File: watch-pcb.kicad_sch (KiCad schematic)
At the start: 104 parts, among them J2 Micro_SD_Card, J3 Conn_01x06_Socket, J4 USB_C_Receptacle, J5 ESP_ANT, U1 LIS3MDL, U10 MX25LM51245GXDI00, U2 BQ25629RYKR, U3 DRV2605LYZFR, U4 BQ27427YZFR, U5 APS12808L-3OBMx, U6 MAX30102, U7 LSM6DSV16XTR, U8 ESP32-S3, Y1 40MHz(10ppm), Y2 32.768kHz

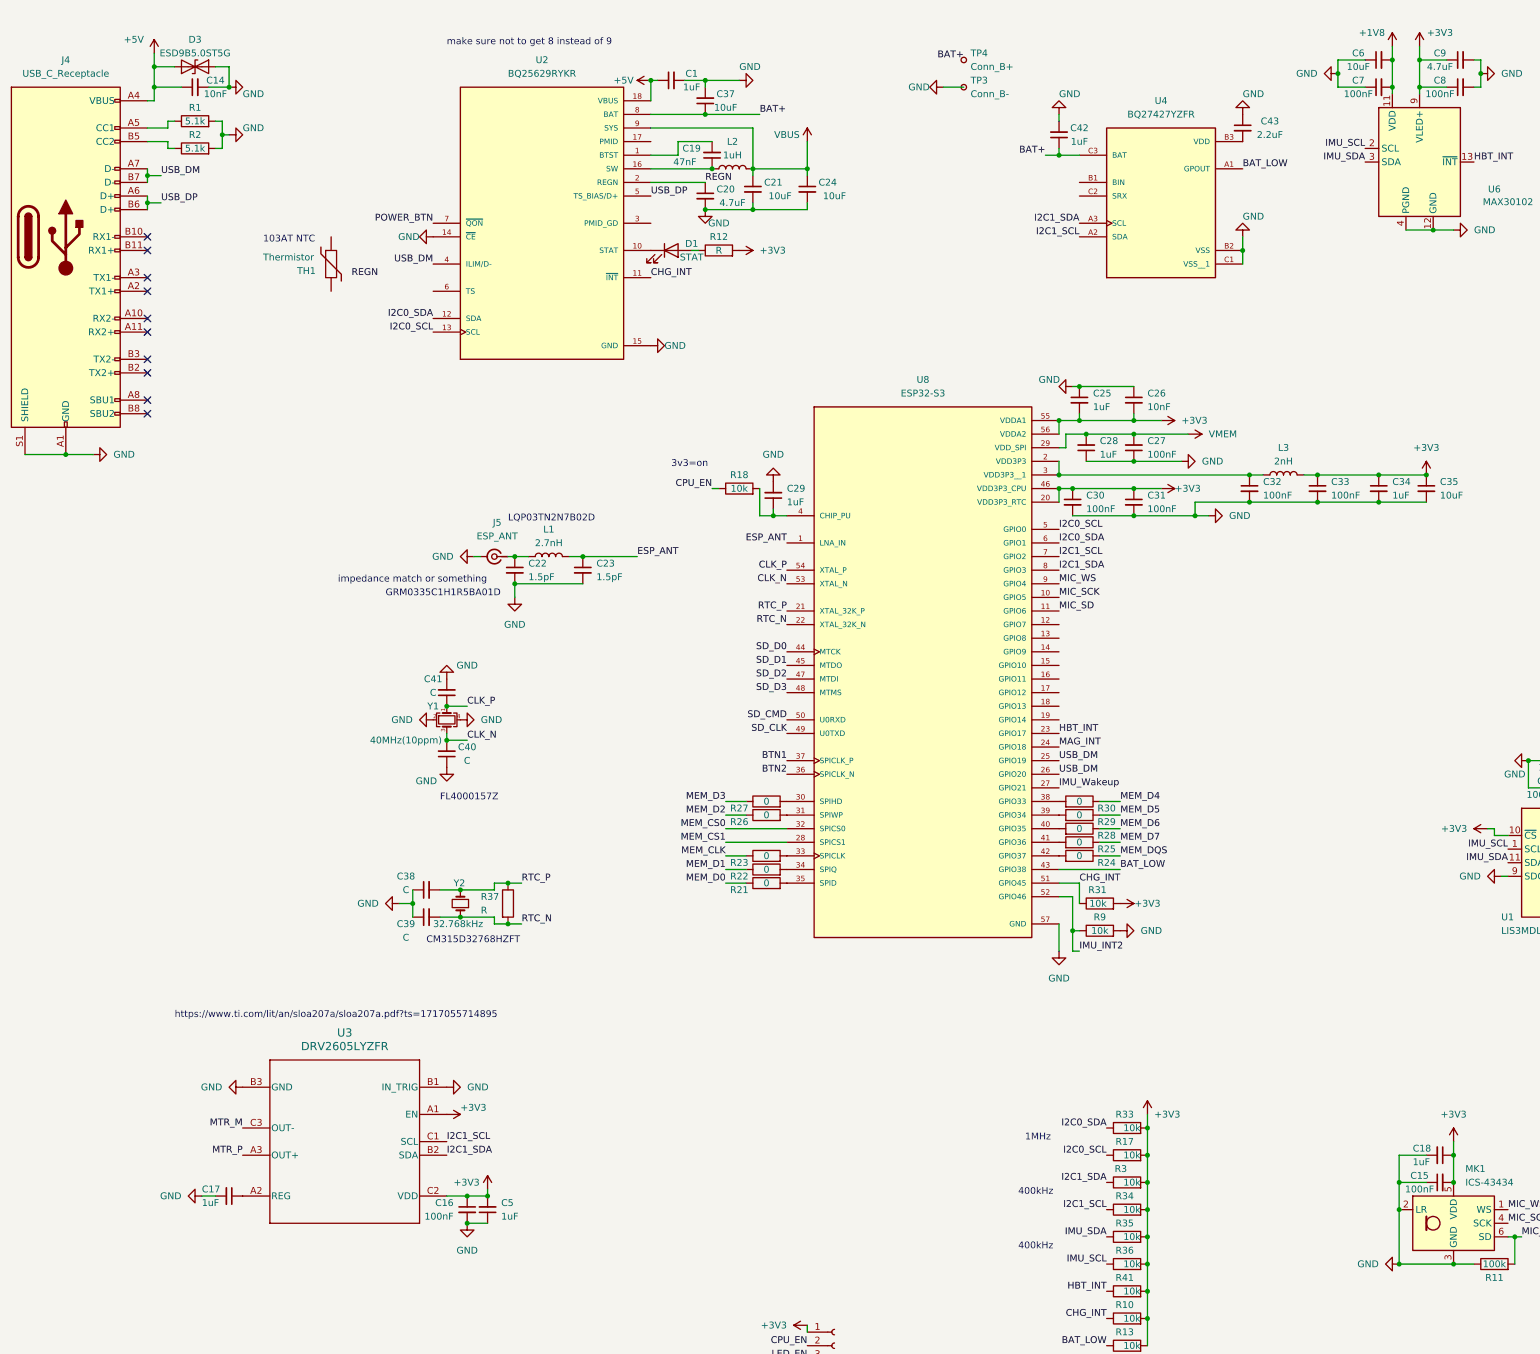
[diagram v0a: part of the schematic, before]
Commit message: display started
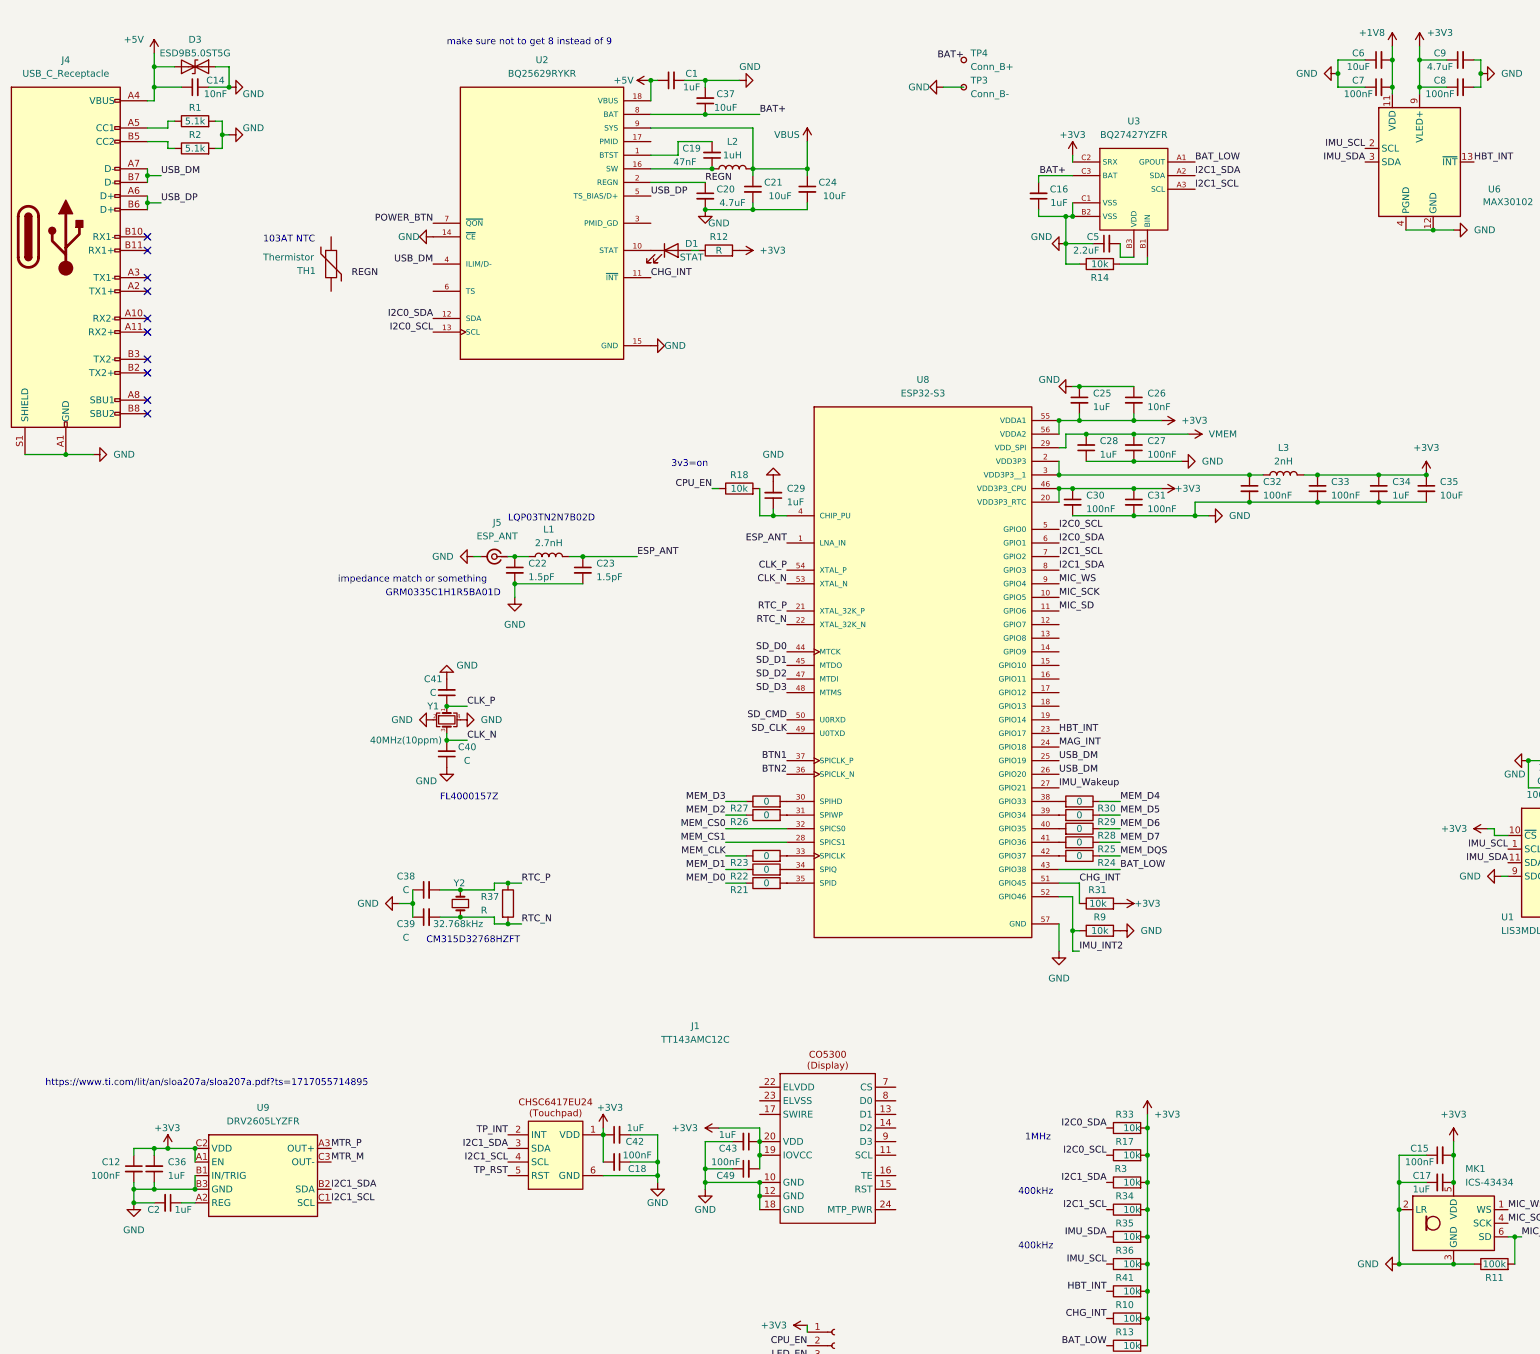
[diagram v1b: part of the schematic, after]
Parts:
- removed U3: DRV2605LYZFR, DRV2605L:YZF0009ADAD, symbol DRV2605LYZFR:DRV2605LYZFR
- removed U4: BQ27427YZFR, BQ27427YZFR:IC_BQ27427YZFR, symbol BQ27427YZFR:BQ27427YZFR
- added C12, C49: 100nF, Capacitor_SMD:C_0201_0603Metric, symbol Device:C_Small
- added C2, C36: 1uF, Capacitor_SMD:C_0201_0603Metric, symbol Device:C_Small
- added J1: TT143AMC12C, symbol custom-lib:TT143AMC12C
- added R14: 10k, symbol Device:R
- added U3: BQ27427YZFR, Package_BGA:Texas_DSBGA-9_1.4715x1.4715mm_Layout3x3_P0.5mm, symbol custom-lib:BQ27427YZFR
- added U9: DRV2605LYZFR, Package_BGA:Texas_DSBGA-9_1.4715x1.4715mm_Layout3x3_P0.5mm, symbol custom-lib:DRV2605LYZFR
- C16: value 100nF -> 1uF
- C18: value 1uF -> 100nF
- C43: value 2.2uF -> 1uF
- C5: value 1uF -> 2.2uF
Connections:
- net +3V3: now also C17.1, C18.2, C42.1, C43.1, C12.1, C36.2, C49.2, J1.1 (VDD), J1.19 (IOVCC), J1.20 (VDD), U3.C2 (SRX), U9.A1 (EN), U9.C2 (VDD); no longer C16.1, C18.1, C5.2
- net BAT+: now also C16.2, U3.C3 (BAT); no longer C42.1
- net BAT_LOW: now also U3.A1 (GPOUT)
- net GND: now also C16.1, C18.1, C43.2, C12.2, C2.2, C36.1, C49.1, J1.10 (GND), J1.12 (GND), J1.18 (GND), J1.6 (GND), R14.1, U3.B2 (VSS), U3.C1 (VSS), U9.B1 (IN/TRIG), U9.B3 (GND); no longer C16.2, C18.2, C43.1
- net I2C1_SCL: now also J1.4 (SCL), U3.A3 (SCL), U9.C1 (SCL)
- net I2C1_SDA: now also J1.3 (SDA), U3.A2 (SDA), U9.B2 (SDA)
- net MTR_M: now also U9.C3 (OUT-)
- net MTR_P: now also U9.A3 (OUT+)
- new net: R14.2, U3.B1 (BIN)
- new net: C2.1, U9.A2 (REG)
- new net: C5.2, U3.B3 (VDD)
- new net TP_INT: J1.2 (INT)
- new net TP_RST: J1.5 (RST)
